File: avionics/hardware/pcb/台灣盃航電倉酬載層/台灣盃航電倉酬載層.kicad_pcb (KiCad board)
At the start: 2 copper layers, 80 x 80 mm, 49 parts, among them U1 MPXV2202DPT1, U10 INA333xxDGK, U2 LM2733YMF, U3 Connector, U4 INA333xxDGK, U5 MPXV2202DPT1, U6 INA333xxDGK, U7 MPXV2202DPT1, U8 INA333xxDGK, U9 MPXV2202DPT1

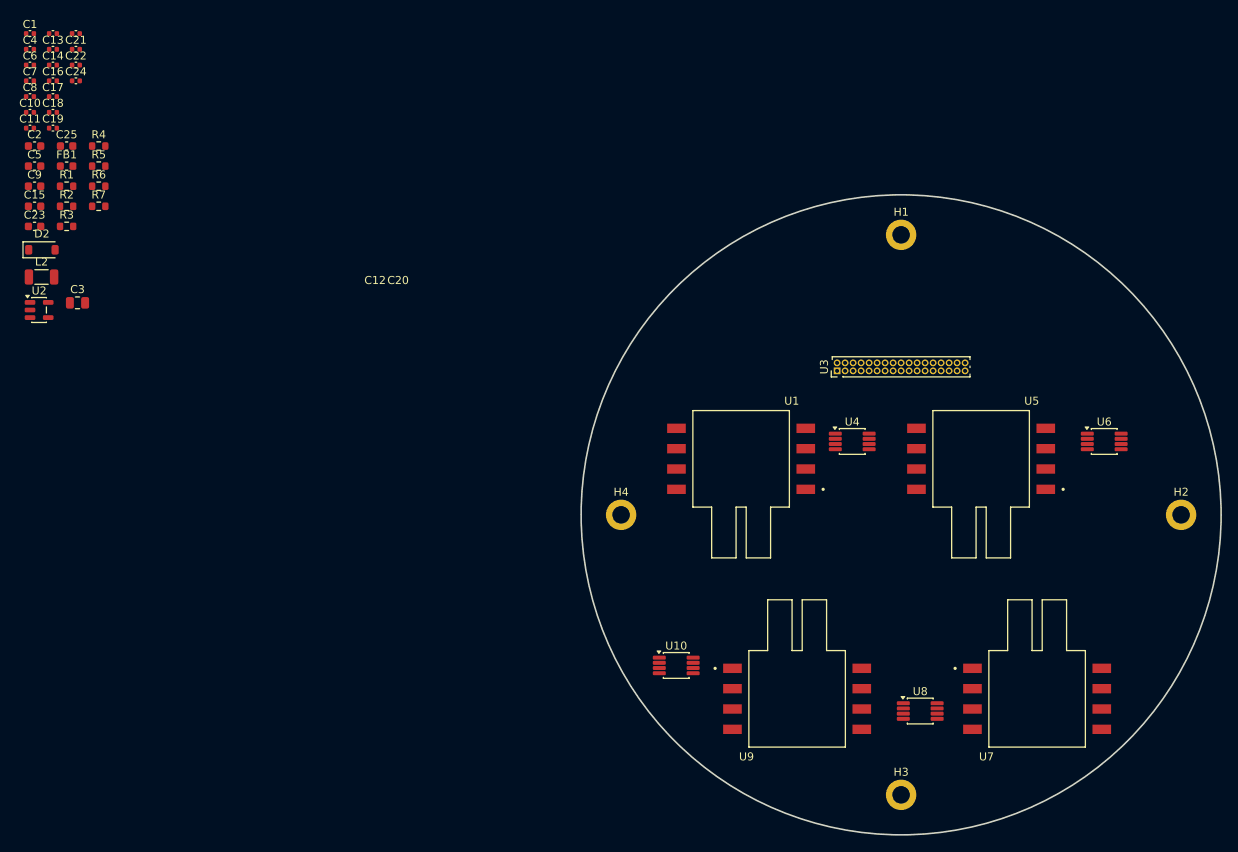
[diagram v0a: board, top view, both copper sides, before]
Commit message: 完成所有航電板設計
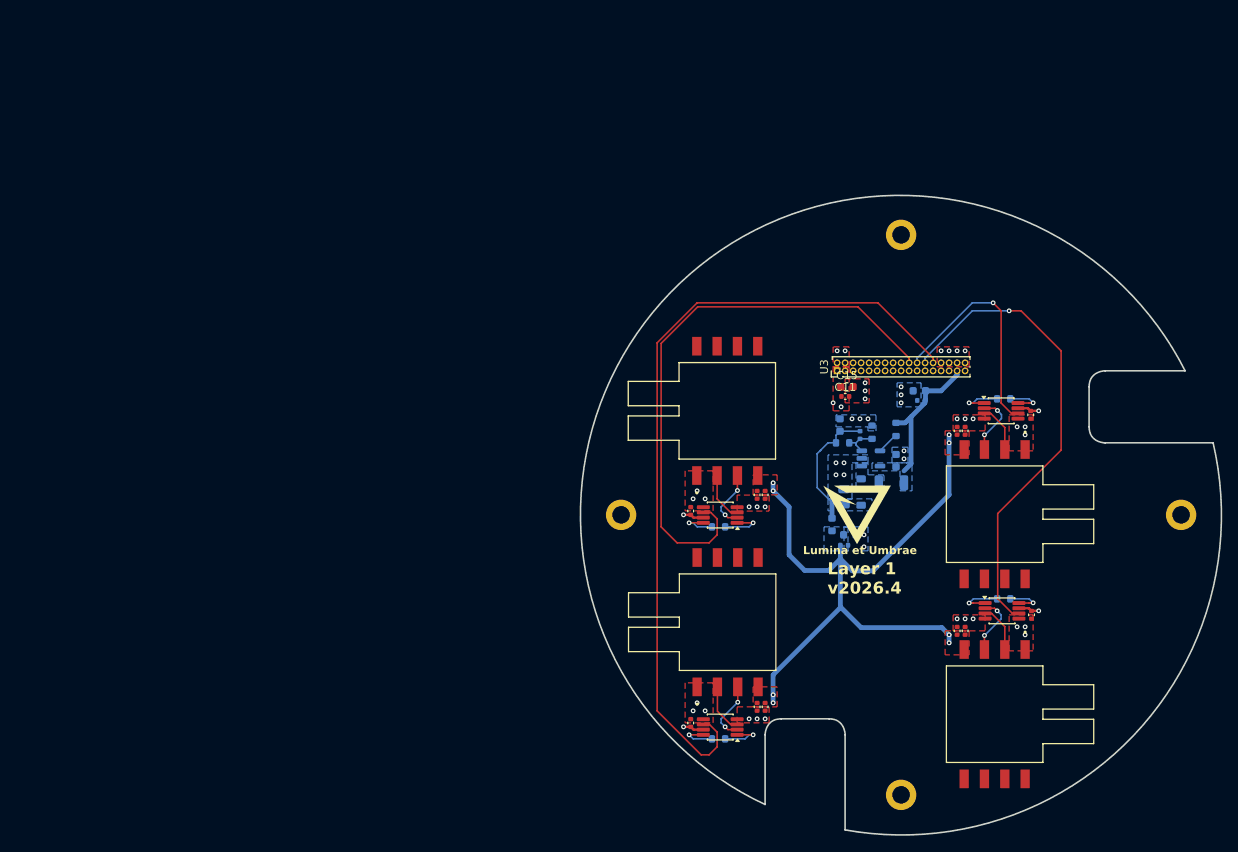
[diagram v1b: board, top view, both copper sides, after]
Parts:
- removed C19: 100n, Capacitor_SMD:C_0402_1005Metric
- removed C23: 10u, Capacitor_SMD:C_0603_1608Metric
- added G***: LOGO, Lumina et Umbrae:ISP_Logo, F.Cu at (141.5, 94.8)
- C1, C2, C24, C25, C3, C4, C5, C6, C9, D2, FB1, L2, R1, R2, R3, R4, R5, R6, R7, U2: moved to B.Cu
- moved C16 140.1 mm to (163.3, 108.5), turned to -90 degrees
- moved C17 131.3 mm to (154.0, 110.5), turned to 90 degrees
- moved C12 131.2 mm to (163.2, 83.5), turned to -90 degrees
- moved C18 131.2 mm to (155.0, 110.5), turned to 90 degrees
- moved R5 125.4 mm to (159.8, 106.5)
- moved C14 122.8 mm to (155.0, 85.5), turned to 90 degrees
- moved C13 122.7 mm to (154.0, 85.5), turned to 90 degrees
- moved C21 119.1 mm to (130.0, 120.0), turned to -90 degrees
- moved C6 118.2 mm to (139.9, 99.8)
- moved R4 117.5 mm to (159.8, 81.5)
- moved C22 117.0 mm to (129.0, 120.0), turned to -90 degrees
- moved C20 115.5 mm to (120.7, 122.0), turned to 90 degrees
- moved C1 115.3 mm to (141.9, 86.0), turned to 90 degrees
- moved C4 114.9 mm to (138.4, 94.0), turned to 90 degrees
- moved C9 113.0 mm to (146.4, 89.2), turned to 90 degrees
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- renumbered C16 to C10, C10 to C16
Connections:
- U3 pad 29: +3V3 -> unconnected-(U3-3V3-Pad29)
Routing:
- net PAYLOAD_4: track 0.00 -> 100.2 mm
- net +10V: track 0.00 -> 82.5 mm, vias 0 -> 8
- net PAYLOAD_1: track 0.00 -> 71.4 mm
- net PAYLOAD_3: track 0.00 -> 59.8 mm, vias 0 -> 1
- net PAYLOAD_2: track 0.00 -> 28.5 mm, vias 0 -> 1
- net +5V: track 0.00 -> 18.6 mm
- net Net-(D2-K): track 0.00 -> 16.0 mm
- net +3V3: track 0.00 -> 10.6 mm, vias 0 -> 6
- net -VOUT_4: track 0.00 -> 7.83 mm, vias 0 -> 2
- net -VOUT_2: track 0.00 -> 7.75 mm, vias 0 -> 2
- net -VOUT_3: track 0.00 -> 7.65 mm, vias 0 -> 2
- net -VOUT_1: track 0.00 -> 7.61 mm, vias 0 -> 2
- net Net-(R5-Pad1): track 0.00 -> 6.23 mm, vias 0 -> 1
- net +VOUT_4: track 0.00 -> 6.19 mm
- net +VOUT_1: track 0.00 -> 6.13 mm
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- added copper zone on B.Cu, net +10V
- added copper zone on F.Cu, net +10V
- added copper zone on F.Cu, net +3V3
- added copper zone on In1.Cu, net +3V3
- added copper zone on B.Cu, net +5V
- added copper zone on B.Cu, net GND
- added copper zone on F.Cu, net GND
- added copper zone on In2.Cu, net GND
- added copper zone on B.Cu, net Net-(D2-A)
- added copper zone on B.Cu, net Net-(D2-K)
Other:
- board size 80 x 80 mm -> 80.1 x 79.9 mm
- copper layers 2 -> 4
- board text added: "Layer 1 v2026.4"
